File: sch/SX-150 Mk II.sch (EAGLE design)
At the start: 189 parts, among them IC1 LM358D, IC2 74HC02D, IC3 LM358D, IC4 LM386M-1, IC5 NJU7096, IC6 REG1117, J1 PJ301M, J2 Line In, Q1 2SC2712, Q10 2SC2712, Q11 2SA1162, Q12 2SC2712, Q13 2SC2712, Q14 2SC2712, Q15 2SC2712, Q16 2SC2712, Q17 2SC2712, Q18 2SC2712, Q19 2SC2712, Q2 2SC2712, Q20 2SC2712, Q21 2SC2712, Q22 2SC2712, Q23 2SC2712, Q24 2SA1162, Q25 2SC2712, Q26 2SC2712, Q27 2SC2712, Q28 2SC2712, Q3 2SC2712, Q4 2SC2712, Q5 2SC2712, Q6 2SC2712, Q7 2SC2712, Q8 2SA1162, Q9 2SC2712, SW1 SP3T, T1 50k, X2 Speaker Out

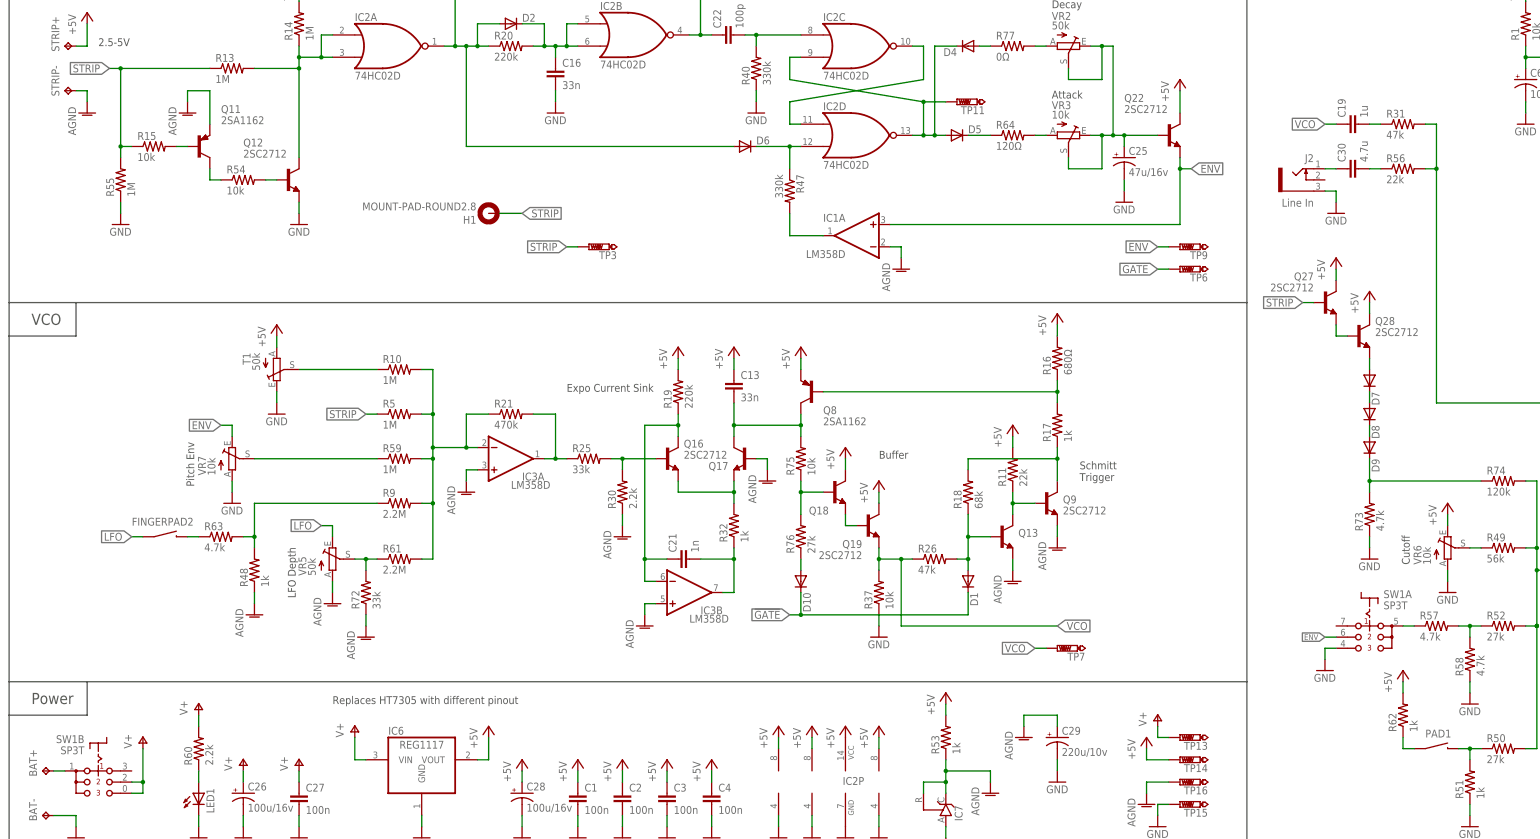
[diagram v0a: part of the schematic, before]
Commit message: Updating board layout and adding gerbers
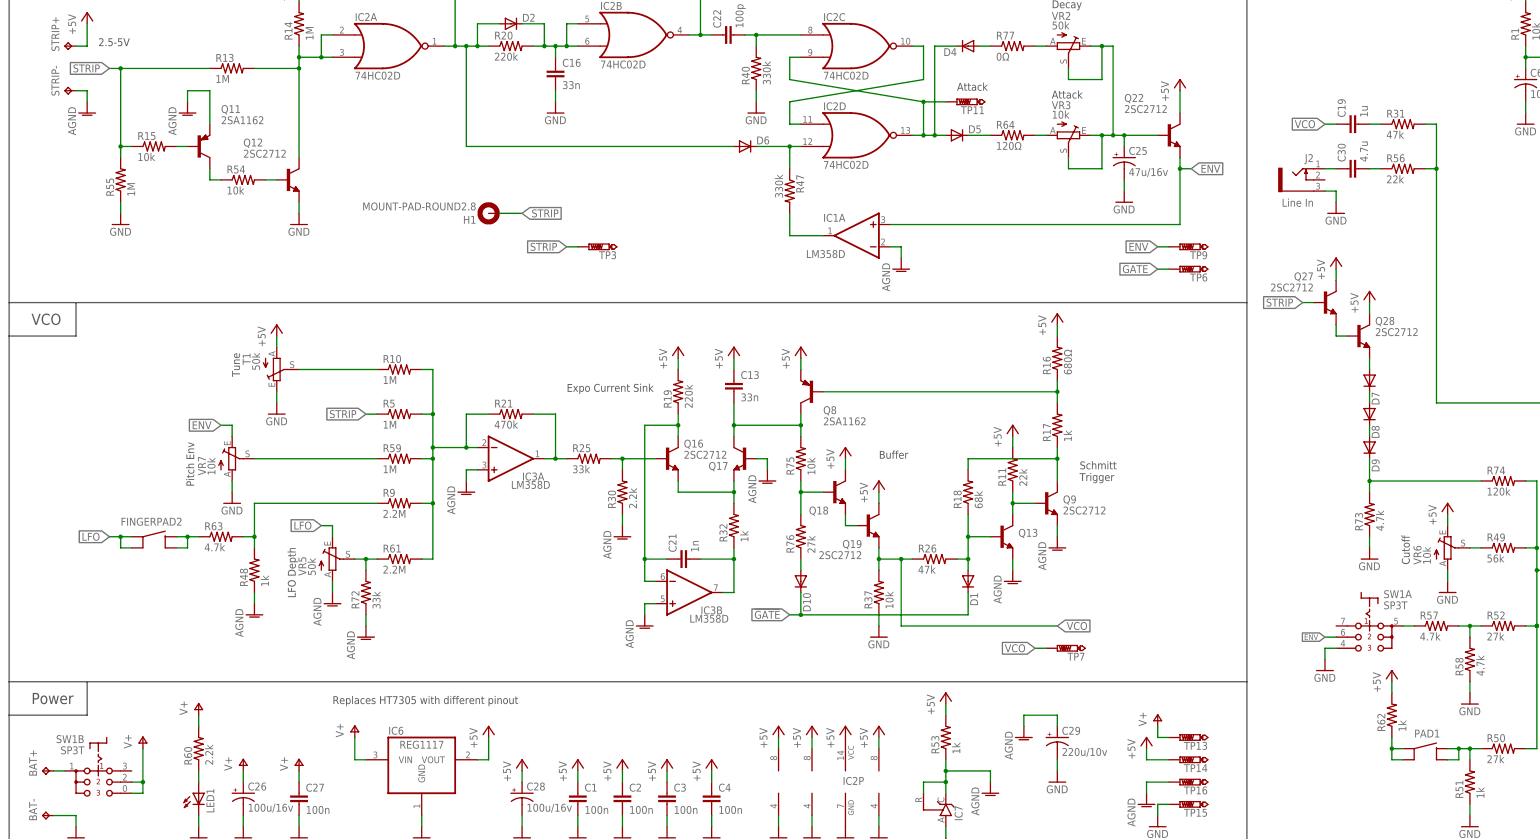
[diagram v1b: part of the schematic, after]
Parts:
- FINGERPAD2, PAD1: value FINGERPAD-2A -> GAKKEN-PAD; device dom-key:FINGERPAD-2A -> dom-key:GAKKEN-PAD
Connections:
- net LFO: now also FINGERPAD2.A0, FINGERPAD2.A1; no longer FINGERPAD2.1
- net N$67: now also PAD1.B0, PAD1.B1; no longer PAD1.2
- net N$77: now also PAD1.A0, PAD1.A1; no longer PAD1.1
- net N$82: now also FINGERPAD2.B0, FINGERPAD2.B1; no longer FINGERPAD2.2
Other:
- note added: "Tune"
- moved on the sheet: R62
